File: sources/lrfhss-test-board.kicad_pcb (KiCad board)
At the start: 2 copper layers, 80.6 x 79 mm, 19 parts, among them J1 SSW-103-01-L-S, J10 SSW-103-01-L-S, J11 SSW-103-01-L-S, J12 SSW-103-01-L-S, J13 09665526616, J2 SSW-103-01-L-S, J3 SSW-103-01-L-S, J4 SSW-103-01-L-S, J5 SSW-103-01-L-S, J6 SSW-103-01-L-S, J7 SSW-103-01-L-S, J8 SSW-103-01-L-S, J9 SSW-103-01-L-S

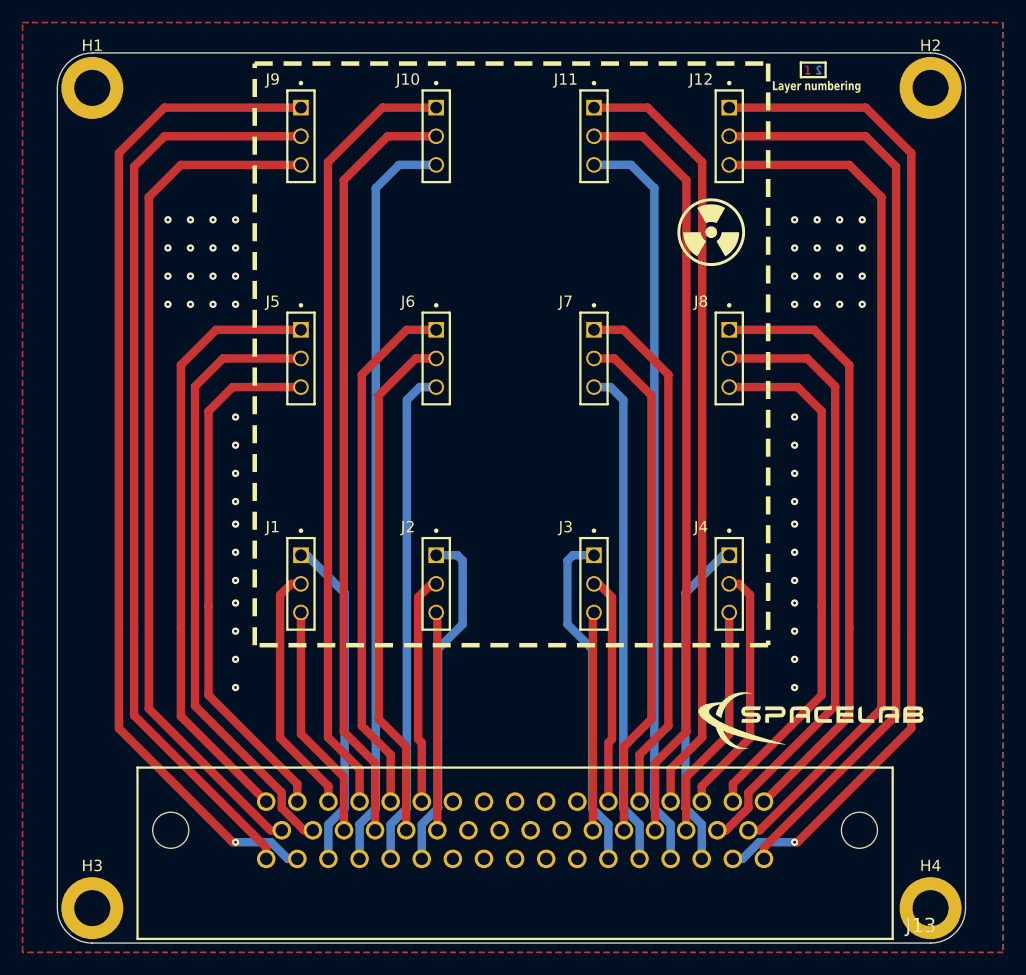
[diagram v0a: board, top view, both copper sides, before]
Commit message: feat: add initial version of the schematic
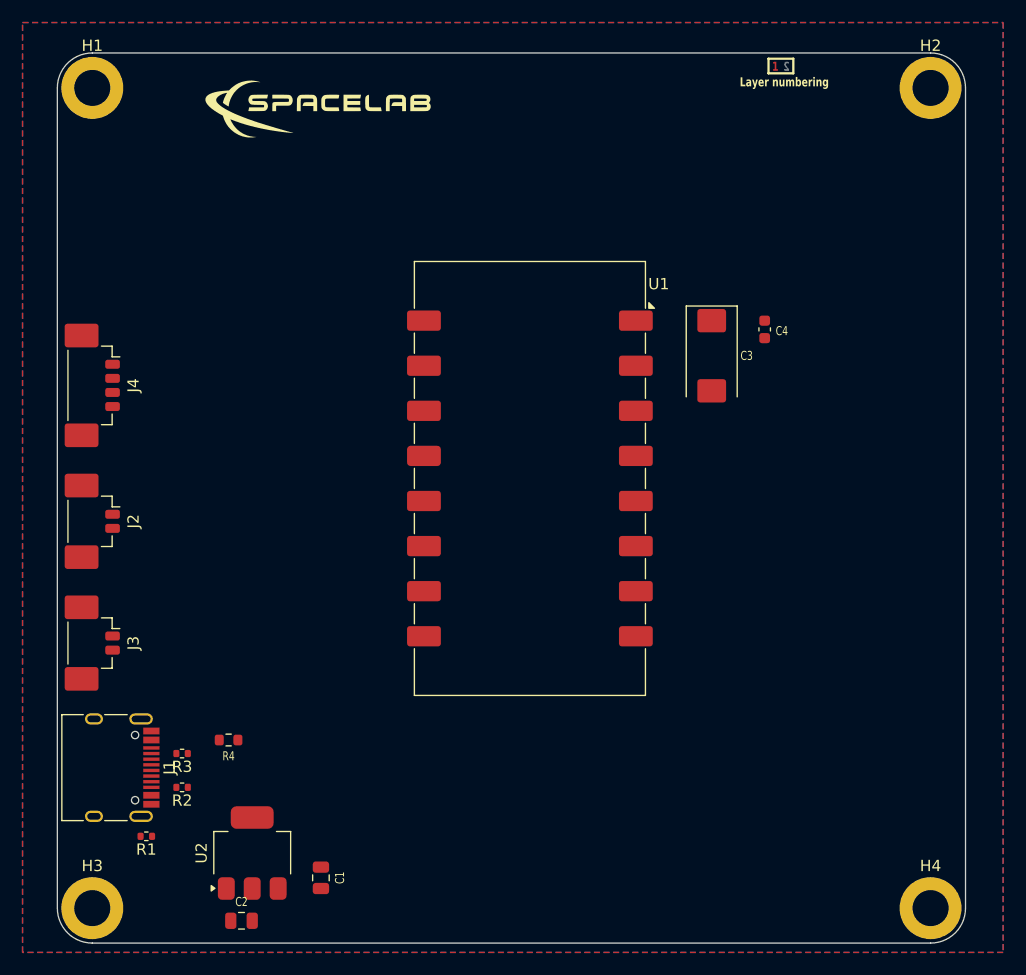
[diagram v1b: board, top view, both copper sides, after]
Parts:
- removed the G*** at (97.3, 54.0)
- removed J10, J11, J12, J5, J6, J7, J8, J9: SSW-103-01-L-S, footprints:SSW-103-01-L-S
- removed J13: 09665526616, footprints:966552616
- added C1: 1uF, footprints:CAP0805, F.Cu at (62.7, 111.3)
- added C2: 1uF, footprints:CAP0805, F.Cu at (55.7, 115.1)
- added C3: 47uF, footprints:CAP2917POL, F.Cu at (97.4, 65.0)
- added C4: 100nF, footprints:CAP0603, F.Cu at (102.1, 62.6)
- added R1: 1M, footprints:RES0402, F.Cu at (47.2, 107.6)
- added R2: 5.11k, footprints:RES0402, F.Cu at (50.4, 103.3)
- added R3: 5.11k, footprints:RES0402, F.Cu at (50.4, 100.3)
- added R4: 1k, footprints:RES0603, F.Cu at (54.5, 99.1)
- added U1: LoRa126XF30, footprints:LoRa126XF30, F.Cu at (81.3, 75.9)
- added U2: AMS1117-3.3, Package_TO_SOT_SMD:SOT-223-3_TabPin2, F.Cu at (56.6, 109.1)
- J1: value SSW-103-01-L-S -> USB-C; footprint footprints:SSW-103-01-L-S -> Connector_USB:USB_C_Receptacle_HRO_TYPE-C-31-M-12
- J2, J3: value SSW-103-01-L-S -> Molex_PicoBlade_53398-0271_1x02-1MP_P1.25mm_Vertical; footprint footprints:SSW-103-01-L-S -> footprints:532610271
- J4: value SSW-103-01-L-S -> Molex_PicoBlade_53398-0471_1x04-1MP_P1.25mm_Vertical; footprint footprints:SSW-103-01-L-S -> footprints:532610471
- moved G*** 69.7 mm to (62.5, 43.1)
- moved J4 58.0 mm to (43.0, 67.6)
- moved J3 44.6 mm to (43.0, 90.5)
- moved J2 30.1 mm to (43.0, 79.7)
- moved J1 25.6 mm to (43.6, 101.5)
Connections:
- J2 pad 1: /V_{G2} -> /CTRL0
- J2 pad 2: /V_{D2} -> /CTRL1
- J2 pad 3: /V_{S2} -> unconnected-(J2-MNTF-Pad3)
- J3 pad 1: /V_{G3} -> /DATA0
- J3 pad 2: /V_{D3} -> /DATA1
- J3 pad 3: /V_{S3} -> unconnected-(J3-MNTF-Pad3)
- J4 pad 1: /V_{G4} -> /SPI0
- J4 pad 2: /V_{D4} -> /SPI1
- J4 pad 3: /V_{S4} -> /SPI2
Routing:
- net /V_{G9}: track 89.5 -> 0.00 mm, vias 1 -> 0
- net /V_{G12}: track 89.5 -> 0.00 mm, vias 1 -> 0
- net /V_{D9}: track 82.2 -> 0.00 mm
- net /V_{D12}: track 82.2 -> 0.00 mm
- net /V_{S12}: track 76.3 -> 0.00 mm
- net /V_{S9}: track 76.3 -> 0.00 mm
- net /V_{G10}: track 69.5 -> 0.00 mm
- net /V_{G11}: track 69.5 -> 0.00 mm
- net /V_{D10}: track 68.6 -> 0.00 mm
- net /V_{D11}: track 68.6 -> 0.00 mm
- net /V_{S10}: track 66.3 -> 0.00 mm
- net /V_{S11}: track 66.3 -> 0.00 mm
- net /V_{D5}: track 54.6 -> 0.00 mm
- net /V_{D8}: track 54.6 -> 0.00 mm
- net /V_{G5}: track 53.8 -> 0.00 mm
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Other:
- board text removed: "V_{D10}"
- board text removed: "V_{D11}"
- board text removed: "V_{D12}"
- board text removed: "V_{D1}"
- board text removed: "V_{D2}"
- board text removed: "V_{D3}"
- board text removed: "V_{D4}"
- board text removed: "V_{D5}"
- board text removed: "V_{D6}"
- board text removed: "V_{D7}"
- board text removed: "V_{D8}"
- board text removed: "V_{D9}"
- board text removed: "V_{G10}"
- board text removed: "V_{G11}"
- board text removed: "V_{G12}"
- board text removed: "V_{G1}"
- board text removed: "V_{G2}"
- board text removed: "V_{G3}"
- board text removed: "V_{G4}"
- board text removed: "V_{G5}"
- board text removed: "V_{G6}"
- board text removed: "V_{G7}"
- board text removed: "V_{G8}"
- board text removed: "V_{G9}"
- board text removed: "V_{S10}"
- board text removed: "V_{S11}"
- board text removed: "V_{S12}"
- board text removed: "V_{S1}"
- board text removed: "V_{S2}"
- board text removed: "V_{S3}"
- board text removed: "V_{S4}"
- board text removed: "V_{S5}"
- board text removed: "V_{S6}"
- board text removed: "V_{S7}"
- board text removed: "V_{S8}"
- board text removed: "V_{S9}"

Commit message: feat: improve schematic and layout
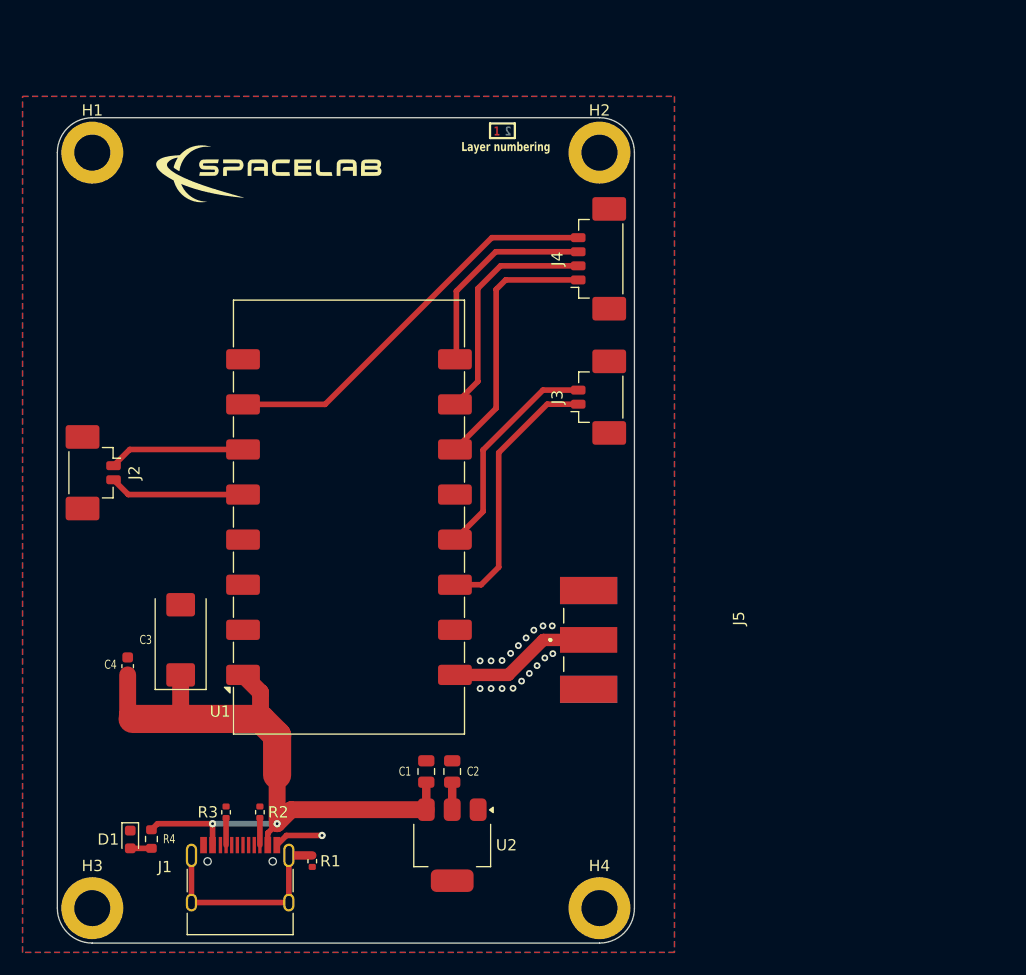
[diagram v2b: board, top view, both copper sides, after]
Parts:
- added D1: LED, LED_SMD:LED_0603_1608Metric, F.Cu at (45.8, 107.9)
- added J5: CINCH_142-0701-801, footprints:142-0701-801, F.Cu at (86.5, 90.2)
- J1: footprint Connector_USB:USB_C_Receptacle_HRO_TYPE-C-31-M-12 -> footprints:GENERIC-USB-C
- J2, J3: value Molex_PicoBlade_53398-0271_1x02-1MP_P1.25mm_Vertical -> 532610271
- J4: value Molex_PicoBlade_53398-0471_1x04-1MP_P1.25mm_Vertical -> 532610471
- moved C4 63.9 mm to (45.6, 92.5), turned to -90 degrees
- moved C3 53.4 mm to (50.3, 90.2), turned to 90 degrees
- moved J3 48.9 mm to (86.8, 68.7), turned to 90 degrees
- moved J4 45.2 mm to (86.8, 56.4), turned to 90 degrees
- moved H2 29.9 mm to (87.4, 47.0)
- moved H4 29.4 mm to (87.4, 114.0)
- moved C2 22.9 mm to (74.4, 101.9), turned to -90 degrees
- moved U2 17.8 mm to (74.4, 108.4), turned to -90 degrees
- moved U1 16.4 mm to (65.2, 79.3), turned to 90 degrees
- moved J1 16.2 mm to (55.5, 112.4), turned to 0 degrees
- moved R1 14.9 mm to (61.9, 109.8), turned to 90 degrees
- moved C1 13.3 mm to (72.1, 101.9)
- moved R4 11.1 mm to (47.7, 107.9), turned to 90 degrees
- moved R2 7.25 mm to (57.3, 105.5), turned to -90 degrees
- moved G*** 7.22 mm to (58.1, 48.8)
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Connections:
- J2 pad 1: /CTRL0 -> /CTRL1
- J2 pad 2: /CTRL1 -> /CTRL0
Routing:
- net VBUS: track 0.00 -> 65.6 mm, vias 0 -> 2
- net /SPI3: track 0.00 -> 35.9 mm
- net /DATA0: track 0.00 -> 23.5 mm
- net /SPI0: track 0.00 -> 23.3 mm
- net /SPI1: track 0.00 -> 20.9 mm
- net /DATA1: track 0.00 -> 19.6 mm
- net Net-(J1-SHIELD): track 0.00 -> 19.1 mm
- net /SPI2: track 0.00 -> 18.4 mm
- net ANT: track 0.00 -> 13.1 mm
- net /CTRL1: track 0.00 -> 12.1 mm
- net /CTRL0: track 0.00 -> 12.0 mm
- net GND: track 0.00 -> 4.37 mm, vias 0 -> 19
- net 3V3: track 0.00 -> 2.44 mm
- net Net-(J1-CC2): track 0.00 -> 2.41 mm
- net Net-(J1-CC1): track 0.00 -> 2.40 mm
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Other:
- board size 80.6 x 79 mm -> 51.2 x 73.2 mm
